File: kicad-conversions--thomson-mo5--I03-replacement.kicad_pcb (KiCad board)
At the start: 2 copper layers, 3 parts, among them U1 HM7603_32×8_PROM_THREE-STATE_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, U2 HIGH_PERFORMANCE_E2_CMOS_PLD_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

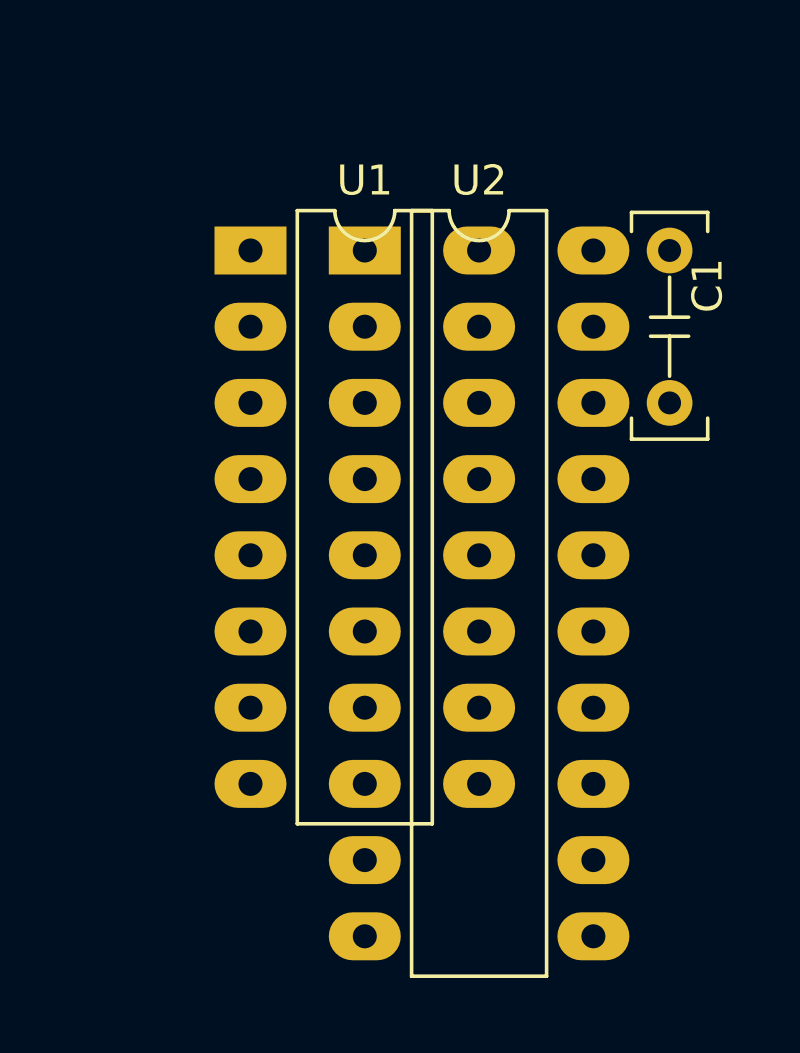
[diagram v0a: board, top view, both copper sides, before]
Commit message: done wiring
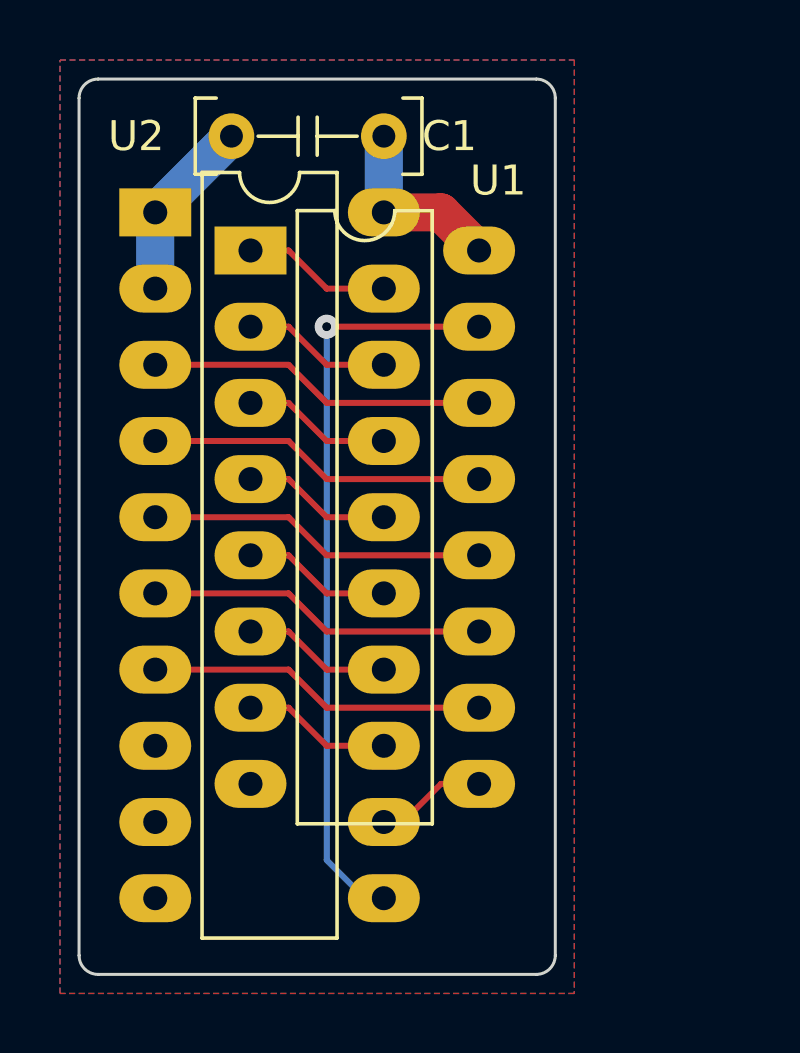
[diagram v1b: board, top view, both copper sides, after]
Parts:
- moved C1 13.6 mm to (78.1, 72.4), turned to 180 degrees
- moved U2 7.10 mm to (73.0, 74.9)
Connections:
- net Net-(U1-GND) renamed /GND
- net Net-(U1-VCC) renamed /VCC
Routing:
- net /~{CE}: track 0.00 -> 25.3 mm, vias 0 -> 1
- net /A1: track 0.00 -> 11.3 mm
- net /A4: track 0.00 -> 11.3 mm
- net /A3: track 0.00 -> 11.3 mm
- net /A2: track 0.00 -> 11.3 mm
- net /A0: track 0.00 -> 11.3 mm
- net /VCC: track 0.00 -> 6.24 mm
- net /GND: track 0.00 -> 6.13 mm
- net /O4: track 0.00 -> 4.97 mm
- net /O2: track 0.00 -> 4.97 mm
- net /O7: track 0.00 -> 4.97 mm
- net /O6: track 0.00 -> 4.97 mm
- net /O5: track 0.00 -> 4.97 mm
- net /O3: track 0.00 -> 4.97 mm
- net /O1: track 0.00 -> 4.97 mm
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- added copper zone on B.Cu, net /GND
- added copper zone on F.Cu, net /GND
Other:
- board outline added: 15.9 x 29.8 mm
